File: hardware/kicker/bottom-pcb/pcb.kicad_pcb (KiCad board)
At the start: 2 copper layers, 45 x 40 mm, 23 parts, among them J1 Conn_01x05, Q1 NMOS, U2 TS4535TP 250GF 009, U4 TC4427AEOA713_C5804606

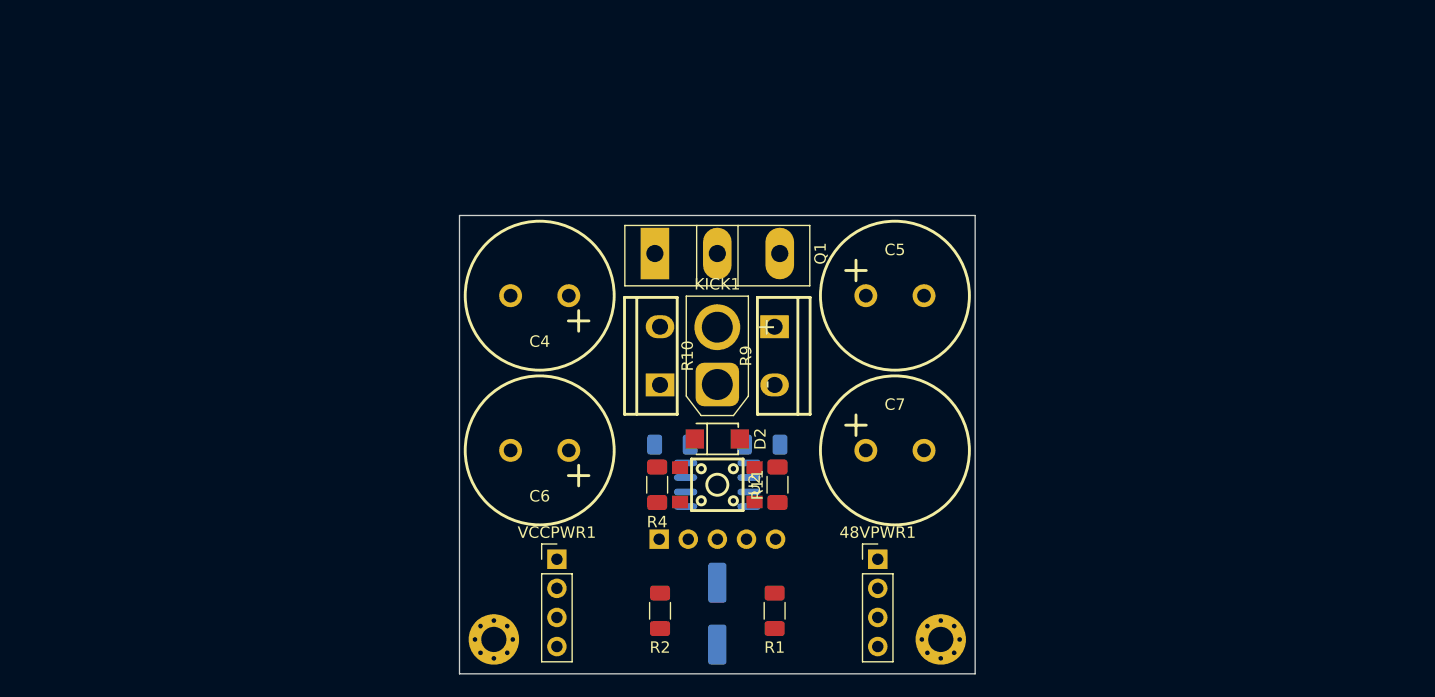
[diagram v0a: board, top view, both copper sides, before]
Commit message: quite a few changes
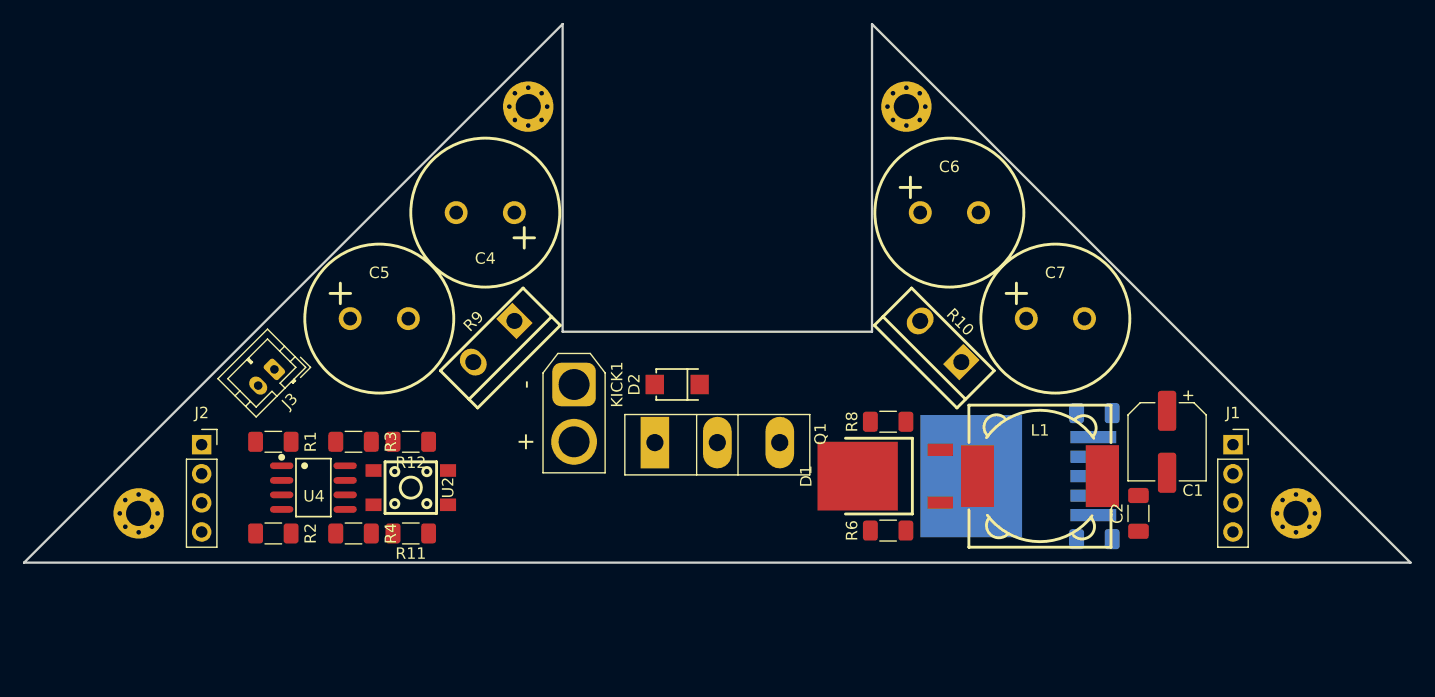
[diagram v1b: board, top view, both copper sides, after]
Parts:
- removed 48VPWR1, VCCPWR1: Conn_01x04, Connector_PinHeader_2.54mm:PinHeader_1x04_P2.54mm_Vertical
- added C2: 1uF, Capacitor_SMD:C_1206_3216Metric_Pad1.33x1.80mm_HandSolder, F.Cu at (36.8, 6.00)
- added C3: 1uF, Capacitor_SMD:C_1206_3216Metric_Pad1.33x1.80mm_HandSolder, B.Cu at (12.2, 2.75)
- added D1: MBRD1045, EasyEDA:TO-252-3_L6.5-W5.9-P4.60-LS10.0-BL, F.Cu at (15.8, 2.75)
- added H3: MountingHole_Pad, MountingHole:MountingHole_2.2mm_M2_Pad_Via, F.Cu at (-50.5, 6.00)
- added H4: MountingHole_Pad, MountingHole:MountingHole_2.2mm_M2_Pad_Via, F.Cu at (50.5, 6.00)
- added J2: Conn_01x04, Connector_PinSocket_2.54mm:PinSocket_1x04_P2.54mm_Vertical, F.Cu at (-45.0, 0.00)
- added J3: Conn_01x02, Connector_JST:JST_PH_B2B-PH-K_1x02_P2.00mm_Vertical, F.Cu at (-38.7, -6.57)
- added L1: SMDRI127-470MT, EasyEDA:IND-SMD_L12.3-W12.3, F.Cu at (28.2, 2.75)
- added R5: 10k, Resistor_SMD:R_1206_3216Metric_Pad1.30x1.75mm_HandSolder, B.Cu at (32.9, -2.75)
- added R6: 73.2kR, Resistor_SMD:R_1206_3216Metric_Pad1.30x1.75mm_HandSolder, F.Cu at (14.9, 7.50)
- added R7: 2kR, Resistor_SMD:R_1206_3216Metric_Pad1.30x1.75mm_HandSolder, B.Cu at (32.9, 8.25)
- added R8: 10kR, Resistor_SMD:R_1206_3216Metric_Pad1.30x1.75mm_HandSolder, F.Cu at (14.9, -2.00)
- added U1: XL6019E1, EasyEDA:TO-263-5_L10.2-W9.9-P1.70-LS14.4-TL, B.Cu at (27.5, 2.75)
- C1, R12, R3, U4: moved to F.Cu
- J1: value Conn_01x05 -> Conn_01x04; footprint Connector_PinHeader_2.54mm:PinHeader_1x05_P2.54mm_Vertical -> Connector_PinSocket_2.54mm:PinSocket_1x04_P2.54mm_Vertical; moved to F.Cu
- moved J1 50.8 mm to (45.0, 0.00), turned to 0 degrees
- moved H1 46.6 mm to (-16.5, -29.5)
- moved H2 46.6 mm to (16.5, -29.5)
- moved R1 46.2 mm to (-38.8, -0.25), turned to 0 degrees
- moved C5 45.0 mm to (-29.5, -11.0)
- moved C1 42.0 mm to (39.2, -0.25), turned to -90 degrees
- moved C6 41.3 mm to (20.2, -20.2), turned to 0 degrees
- moved U4 35.3 mm to (-35.2, 3.75)
- moved R2 34.4 mm to (-38.8, 7.75), turned to 0 degrees
- moved R11 32.3 mm to (-26.8, 7.75), turned to 0 degrees
- moved R12 30.7 mm to (-26.8, -0.25)
- moved R3 27.8 mm to (-31.8, -0.25)
- moved R4 26.8 mm to (-31.8, 7.75), turned to 180 degrees
- moved U2 26.8 mm to (-26.8, 3.75)
- moved R10 24.5 mm to (19.5, -9.00), turned to 135 degrees
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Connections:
- D2 pad 2: /OUTA -> Net-(D2-A)
- J1 pad 1: /OUTB -> VCC
- J1 pad 2: /INB -> VCC
- J1 pad 3: /INA -> GND
- J1 pad 4: VCC -> GND
- KICK1 pad 2: Net-(KICK1-Pin_2) -> Net-(D2-A)
- Q1 pad 1: Net-(KICK1-Pin_2) -> Net-(D2-A)
- R10 pad 1: CAP_VCC -> +48V
- R10 pad 2: +48V -> CAP_VCC
- R9 pad 1: +48V -> CAP_VCC
- R9 pad 2: CAP_VCC -> +48V
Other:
- board size 45 x 40 mm -> 121 x 47 mm
